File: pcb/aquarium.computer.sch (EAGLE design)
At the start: 56 parts, among them K1 JS-M1-9V-4, K2 JS-M1-9V-4, M328 ATMEGA328P-AU, Q1 BC447, Q2 BC447, Q3 BC447, Q4 BC447, Q5 BC447, Q6 BC447

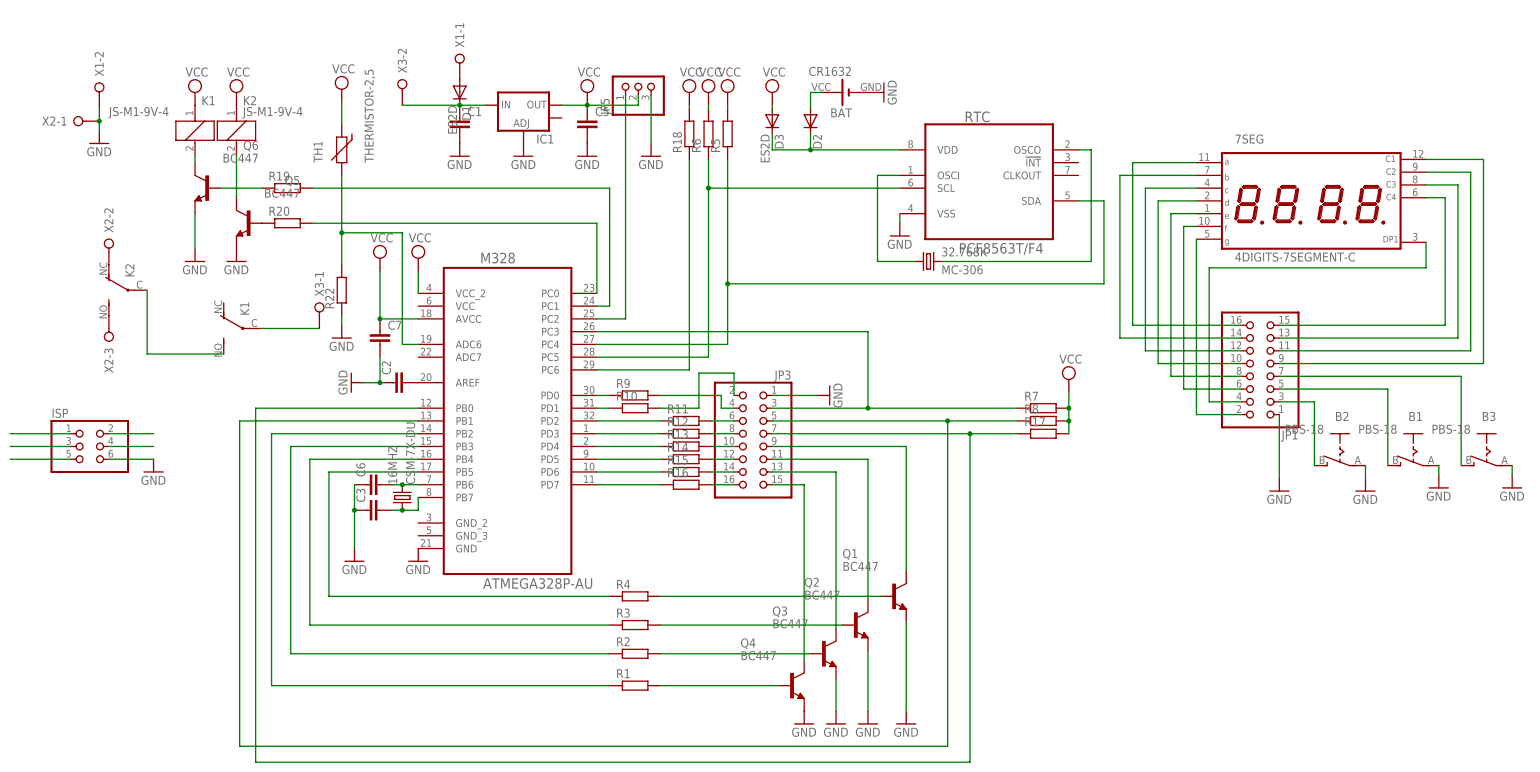
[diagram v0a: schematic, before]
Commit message: thermistor code
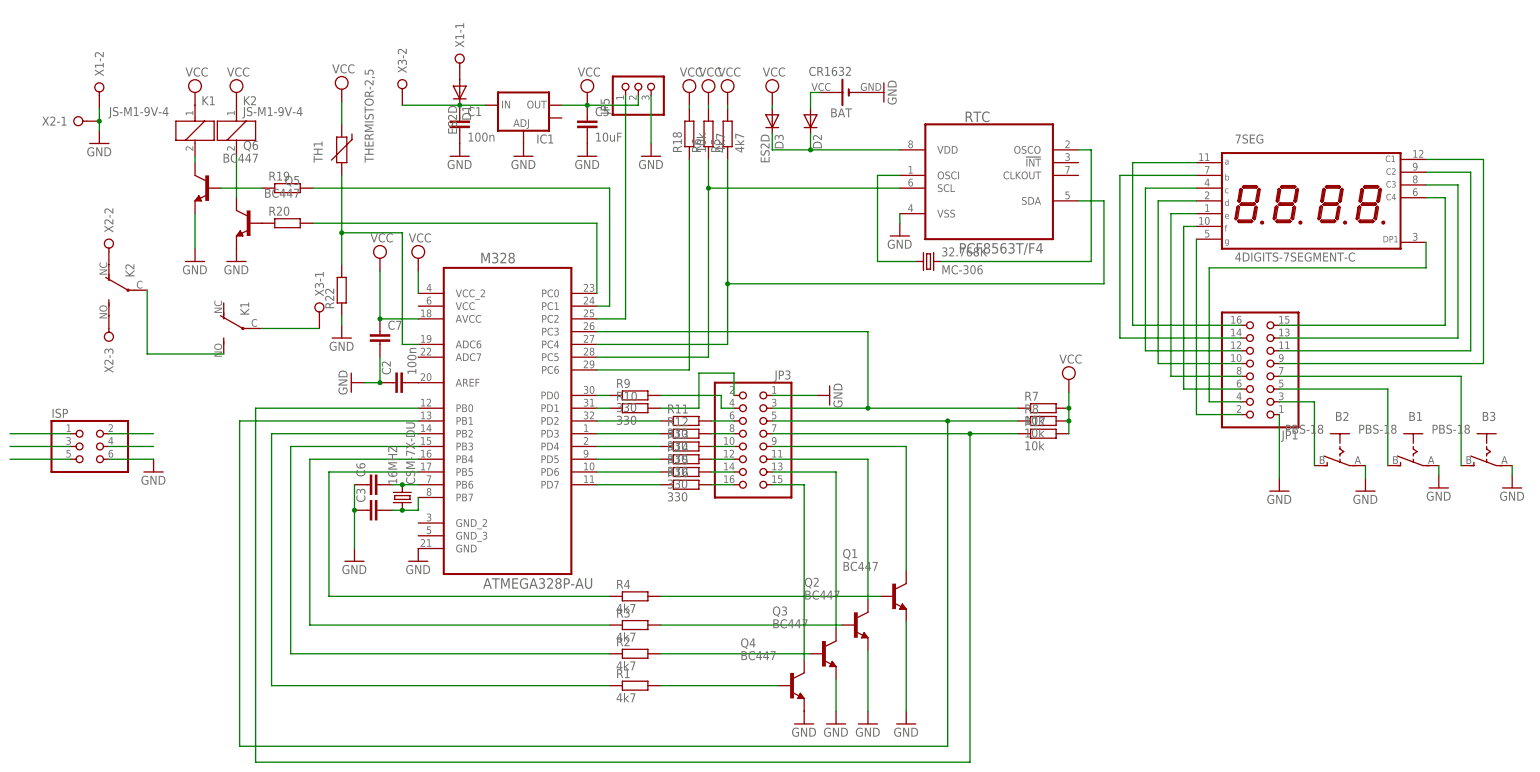
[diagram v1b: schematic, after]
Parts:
- C1, C2: value (none) -> 100n
- C5: value (none) -> 10uF
- R1, R2, R3, R4, R5, R6: value (none) -> 4k7
- R10, R11, R12, R13, R14, R15, R16, R9: value (none) -> 330
- R17, R18, R7, R8: value (none) -> 10k
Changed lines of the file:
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@@
 <setting verticaltext="up"/>
 </settings>
-<grid distance="25" unitdist="mil" unit="mil" style="lines" multiple="1" display="no" altdistance="0.01" altunitdist="inch" altunit="inch"/>
+<grid distance="0.1" unitdist="inch" unit="inch" style="lines" multiple="1" display="no" altdistance="0.01" altunitdist="inch" altunit="inch"/>
 <layers>
 <layer number="1" name="Top" color="4" fill="1" visible="no" active="no"/>
@@
 <layer number="94" name="Symbols" color="4" fill="1" visible="yes" active="yes"/>
 <layer number="95" name="Names" color="7" fill="1" visible="yes" active="yes"/>
-<layer number="96" name="Values" color="7" fill="1" visible="yes" active="yes"/>
+<layer number="96" name="Values" color="7" fill="1" visible="no" active="yes"/>
 <layer number="97" name="Info" color="7" fill="1" visible="yes" active="yes"/>
 <layer number="98" name="Guide" color="6" fill="1" visible="yes" active="yes"/>
@@
 <part name="GND1" library="supply1" deviceset="GND" device=""/>
 <part name="GND2" library="supply1" deviceset="GND" device=""/>
-<part name="R5" library="rcl" deviceset="R-EU_" device="R1206"/>
-<part name="R6" library="rcl" deviceset="R-EU_" device="R1206"/>
+<part name="R5" library="rcl" deviceset="R-EU_" device="R1206" value="4k7"/>
+<part name="R6" library="rcl" deviceset="R-EU_" device="R1206" value="4k7"/>
 <part name="SUPPLY7" library="supply2" deviceset="VCC" device=""/>
 <part name="GND3" library="supply1" deviceset="GND" device=""/>
@@
 <part name="32.768K" library="quarz" deviceset="MC-306" device=""/>
 <part name="JP3" library="pinhead" deviceset="PINHD-2X8" device=""/>
-<part name="R9" library="rcl" deviceset="R-EU_" device="0207/10"/>
-<part name="R10" library="rcl" deviceset="R-EU_" device="0207/10"/>
-<part name="R11" library="rcl" deviceset="R-EU_" device="0207/10"/>
-<part name="R12" library="rcl" deviceset="R-EU_" device="0207/10"/>
-<part name="R13" library="rcl" deviceset="R-EU_" device="0207/10"/>
-<part name="R14" library="rcl" deviceset="R-EU_" device="0207/10"/>
-<part name="R15" library="rcl" deviceset="R-EU_" device="0207/10"/>
-<part name="R16" library="rcl" deviceset="R-EU_" device="0207/10"/>
+<part name="R9" library="rcl" deviceset="R-EU_" device="0207/10" value="330"/>
+<part name="R10" library="rcl" deviceset="R-EU_" device="0207/10" value="330"/>
+<part name="R11" library="rcl" deviceset="R-EU_" device="0207/10" value="330"/>
+<part name="R12" library="rcl" deviceset="R-EU_" device="0207/10" value="330"/>
+<part name="R13" library="rcl" deviceset="R-EU_" device="0207/10" value="330"/>
+<part name="R14" library="rcl" deviceset="R-EU_" device="0207/10" value="330"/>
+<part name="R15" library="rcl" deviceset="R-EU_" device="0207/10" value="330"/>
+<part name="R16" library="rcl" deviceset="R-EU_" device="0207/10" value="330"/>
 <part name="Q1" library="transistor-npn" deviceset="BC447*" device=""/>
 <part name="Q2" library="transistor-npn" deviceset="BC447*" device=""/>
 <part name="Q3" library="transistor-npn" deviceset="BC447*" device=""/>
 <part name="Q4" library="transistor-npn" deviceset="BC447*" device=""/>
-<part name="R7" library="rcl" deviceset="R-EU_" device="0207/10"/>
-<part name="R8" library="rcl" deviceset="R-EU_" device="0207/10"/>
+<part name="R7" library="rcl" deviceset="R-EU_" device="0207/10" value="10k"/>
+<part name="R8" library="rcl" deviceset="R-EU_" device="0207/10" value="10k"/>
 <part name="Q5" library="transistor-npn" deviceset="BC447*" device=""/>
 <part name="Q6" library="transistor-npn" deviceset="BC447*" device=""/>
@@
 <part name="GND15" library="supply1" deviceset="GND" device=""/>
 <part name="GND16" library="supply1" deviceset="GND" device=""/>
-<part name="R17" library="rcl" deviceset="R-EU_" device="0207/10"/>
+<part name="R17" library="rcl" deviceset="R-EU_" device="0207/10" value="10k"/>
 <part name="SUPPLY11" library="supply2" deviceset="VCC" device=""/>
 <part name="SUPPLY12" library="supply2" deviceset="VCC" device=""/>
@@
 <part name="JP1" library="pinhead" deviceset="PINHD-2X8" device=""/>
 <part name="X1" library="con-wago-508" deviceset="W237-02P" device=""/>
-<part name="R1" library="rcl" deviceset="R-EU_" device="0207/10"/>
-<part name="R2" library="rcl" deviceset="R-EU_" device="0207/10"/>
-<part name="R3" library="rcl" deviceset="R-EU_" device="0207/10"/>
-<part name="R4" library="rcl" deviceset="R-EU_" device="0207/10"/>
+<part name="R1" library="rcl" deviceset="R-EU_" device="0207/10" value="4k7"/>
+<part name="R2" library="rcl" deviceset="R-EU_" device="0207/10" value="4k7"/>
+<part name="R3" library="rcl" deviceset="R-EU_" device="0207/10" value="4k7"/>
+<part name="R4" library="rcl" deviceset="R-EU_" device="0207/10" value="4k7"/>
 <part name="TH1" library="varistor" deviceset="THERMISTOR" device="-2,5"/>
 <part name="R22" library="rcl" deviceset="R-EU_" device="R1206"/>
@@
 <part name="R19" library="rcl" deviceset="R-EU_" device="0207/10"/>
 <part name="R20" library="rcl" deviceset="R-EU_" device="0207/10"/>
-<part name="C1" library="rcl" deviceset="C-EU" device="025-040X050"/>
-<part name="R18" library="rcl" deviceset="R-EU_" device="0207/10"/>
-<part name="C5" library="rcl" deviceset="C-EU" device="025-050X050"/>
-<part name="C2" library="rcl" deviceset="C-EU" device="C1206"/>
+<part name="C1" library="rcl" deviceset="C-EU" device="025-040X050" value="100n"/>
+<part name="R18" library="rcl" deviceset="R-EU_" device="0207/10" value="10k"/>
+<part name="C5" library="rcl" deviceset="C-EU" device="025-050X050" value="10uF"/>
+<part name="C2" library="rcl" deviceset="C-EU" device="C1206" value="100n"/>
 <part name="SUPPLY3" library="supply2" deviceset="VCC" device=""/>
 <part name="GND22" library="supply1" deviceset="GND" device=""/>
